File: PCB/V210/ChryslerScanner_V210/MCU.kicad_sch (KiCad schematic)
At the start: 30 parts, among them J1 I2C, Q1 UMH3N, SW1 RESET, SW2 BOOT, U1 ESP32-PICO-D4, U2 AW9523B

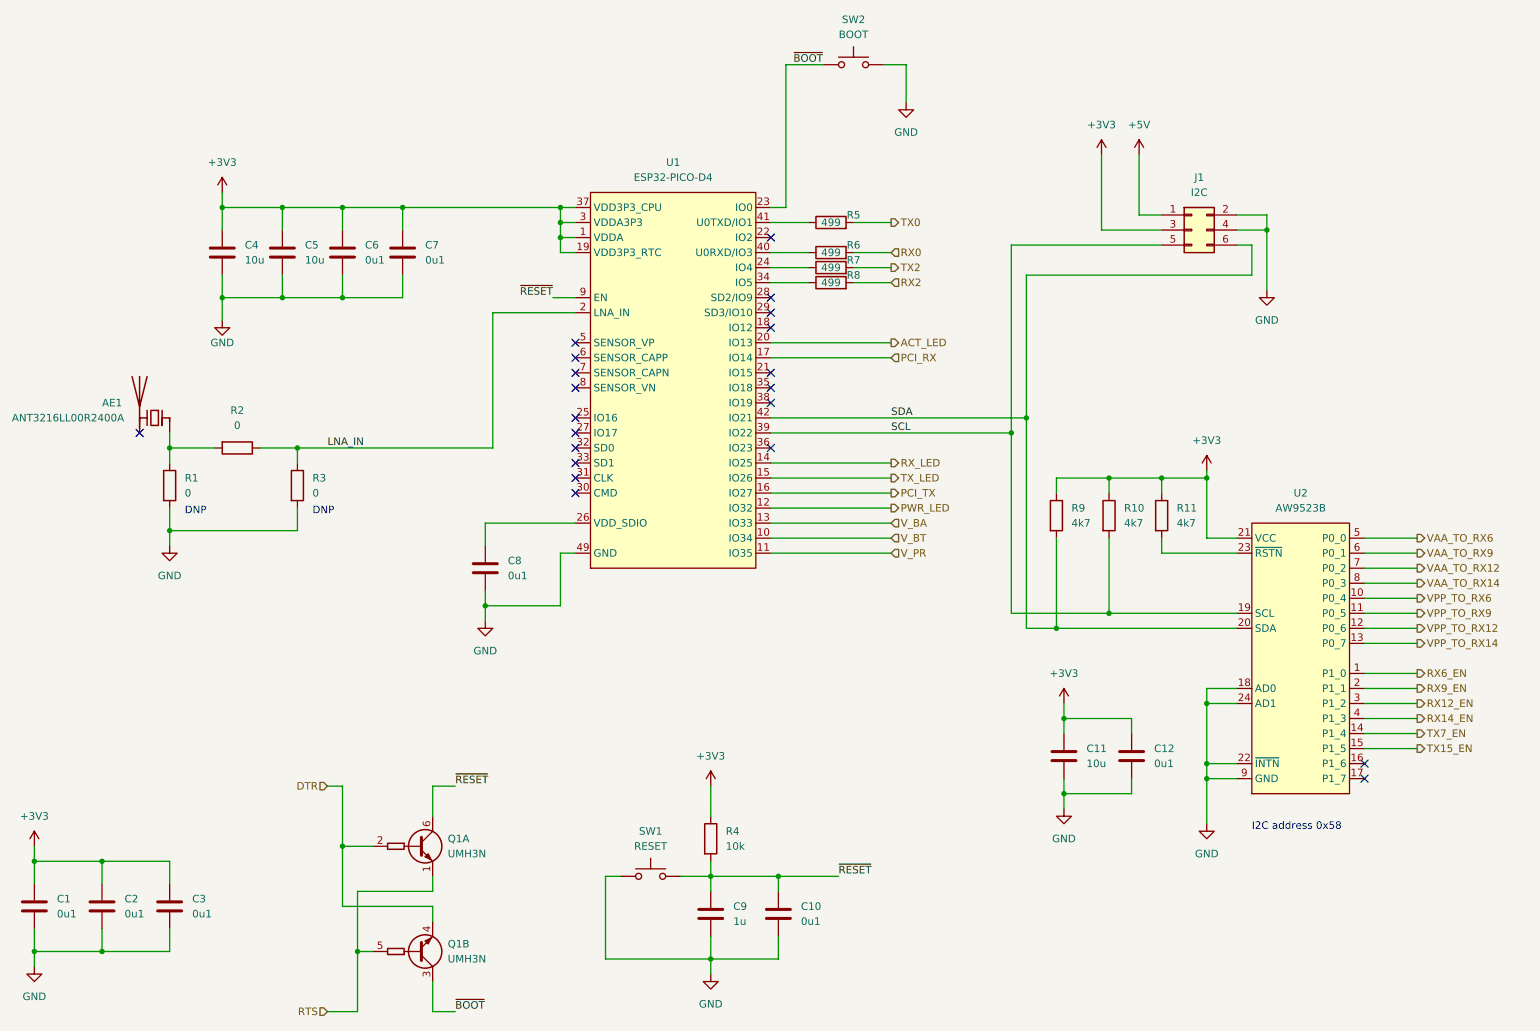
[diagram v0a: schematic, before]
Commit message: WIP
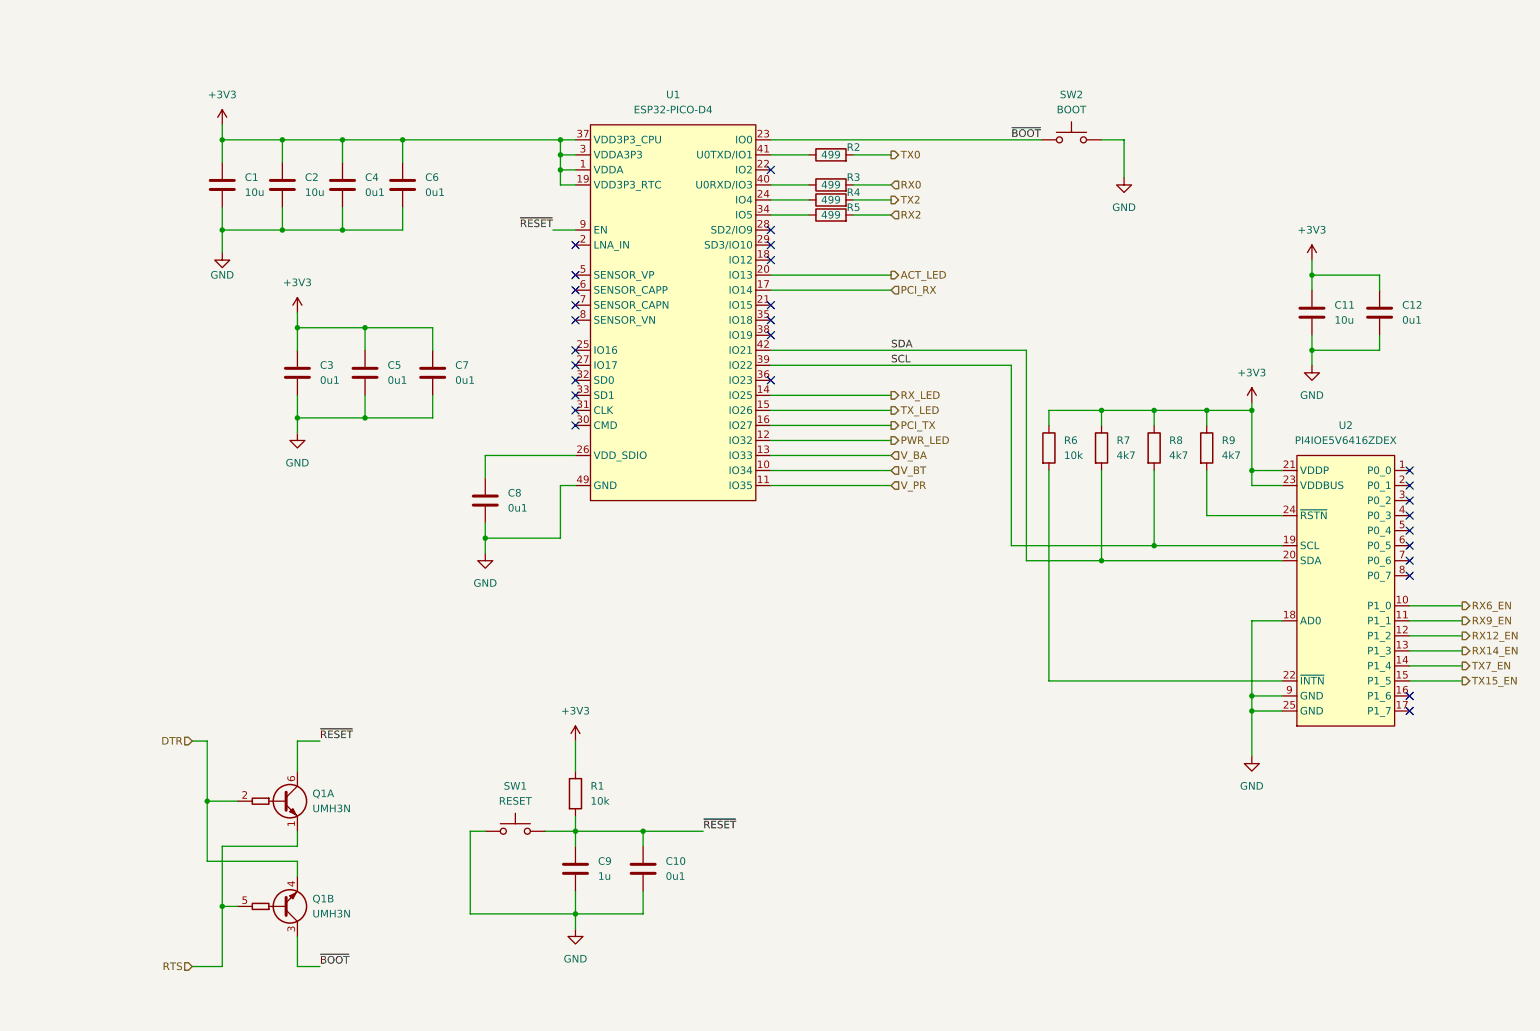
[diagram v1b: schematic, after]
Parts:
- removed AE1: ANT3216LL00R2400A, symbol Device:Antenna_Chip
- removed J1: I2C, symbol Connector_Generic:Conn_02x03_Odd_Even
- removed R1, R2, R3: 0, symbol Device:R
- removed U2: AW9523B, symbol ChryslerScanner:AW9523B
- added R6: 10k, Resistor_SMD:R_0603_1608Metric, symbol Device:R
- added U2: PI4IOE5V6416ZDEX, Package_DFN_QFN:QFN-24-1EP_4x4mm_P0.5mm_EP2.15x2.15mm_ThermalVias, symbol ChryslerScanner:PI4IOE5V6416ZDEX
- C1: renamed from C4; footprint (none) -> Capacitor_SMD:C_0603_1608Metric
- C10, C11, C12, C8, C9: footprint (none) -> Capacitor_SMD:C_0603_1608Metric
- C2: renamed from C5; footprint (none) -> Capacitor_SMD:C_0603_1608Metric
- C3: renamed from C1; footprint (none) -> Capacitor_SMD:C_0603_1608Metric
- C4: renamed from C6; footprint (none) -> Capacitor_SMD:C_0603_1608Metric
- C5: renamed from C2; footprint (none) -> Capacitor_SMD:C_0603_1608Metric
- C6: renamed from C7; footprint (none) -> Capacitor_SMD:C_0603_1608Metric
- C7: renamed from C3; footprint (none) -> Capacitor_SMD:C_0603_1608Metric
- Q1: manf# (none) -> UMH3NTN
- R1: renamed from R4; footprint (none) -> Resistor_SMD:R_0603_1608Metric
- R2: renamed from R5; footprint (none) -> Resistor_SMD:R_0603_1608Metric
- R3: renamed from R6; footprint (none) -> Resistor_SMD:R_0603_1608Metric
- R4: renamed from R7; footprint (none) -> Resistor_SMD:R_0603_1608Metric
- R5: renamed from R8; footprint (none) -> Resistor_SMD:R_0603_1608Metric
- R7: renamed from R9; footprint (none) -> Resistor_SMD:R_0603_1608Metric
- R8: renamed from R10; footprint (none) -> Resistor_SMD:R_0603_1608Metric
- R9: renamed from R11; footprint (none) -> Resistor_SMD:R_0603_1608Metric
- SW1, SW2: footprint (none) -> EmSA:TL6330 Tactile Switch
- U1: footprint (none) -> Package_DFN_QFN:QFN-48-1EP_7x7mm_P0.5mm_EP5.15x5.15mm_ThermalVias; manf# (none) -> ESP32-PICO-D4
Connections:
- net +3V3: now also R6.1, U2.21 (VDDP), U2.23 (VDDBUS)
- net GND: now also U2.18 (AD0), U2.25 (GND), U2.9 (GND)
- net RX12_EN: now also U2.12 (P1_2)
- net RX14_EN: now also U2.13 (P1_3)
- net RX6_EN: now also U2.10 (P1_0)
- net RX9_EN: now also U2.11 (P1_1)
- net SCL: now also U2.19 (SCL)
- net SDA: now also U2.20 (SDA)
- net TX15_EN: now also U2.15 (P1_5)
- net TX7_EN: now also U2.14 (P1_4)
- net at R9.2: now also U2.24 (~{RSTN})
- net LNA_IN: no longer names the net of U1.2 (LNA_IN)
- new net: R6.2, U2.22 (~{INTN})
- no-connect marks 21 -> 29
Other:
- note removed: "DNP"
- note removed: "I2C address 0x58"
- title: Chrysler Scanner -> TJ Diag
- moved on the sheet: C1, C10, C11, C12, C2, C3, C4, C5, C6, C7, C8, C9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
